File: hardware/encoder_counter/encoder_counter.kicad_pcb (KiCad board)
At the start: 2 copper layers, 32 parts, among them P1 5045-3, P2 FEMALE_HEADER, P3 5045-3, P4 5045-3, P5 FEMALE_HEADER, P6 FEMALE_HEADER, P7 5045-3, P8 FEMALE_HEADER, P9 FEMALE_HEADER, U5 LS7366R, U6 LS7366R, Y1 32 MHz, Y2 32 MHz

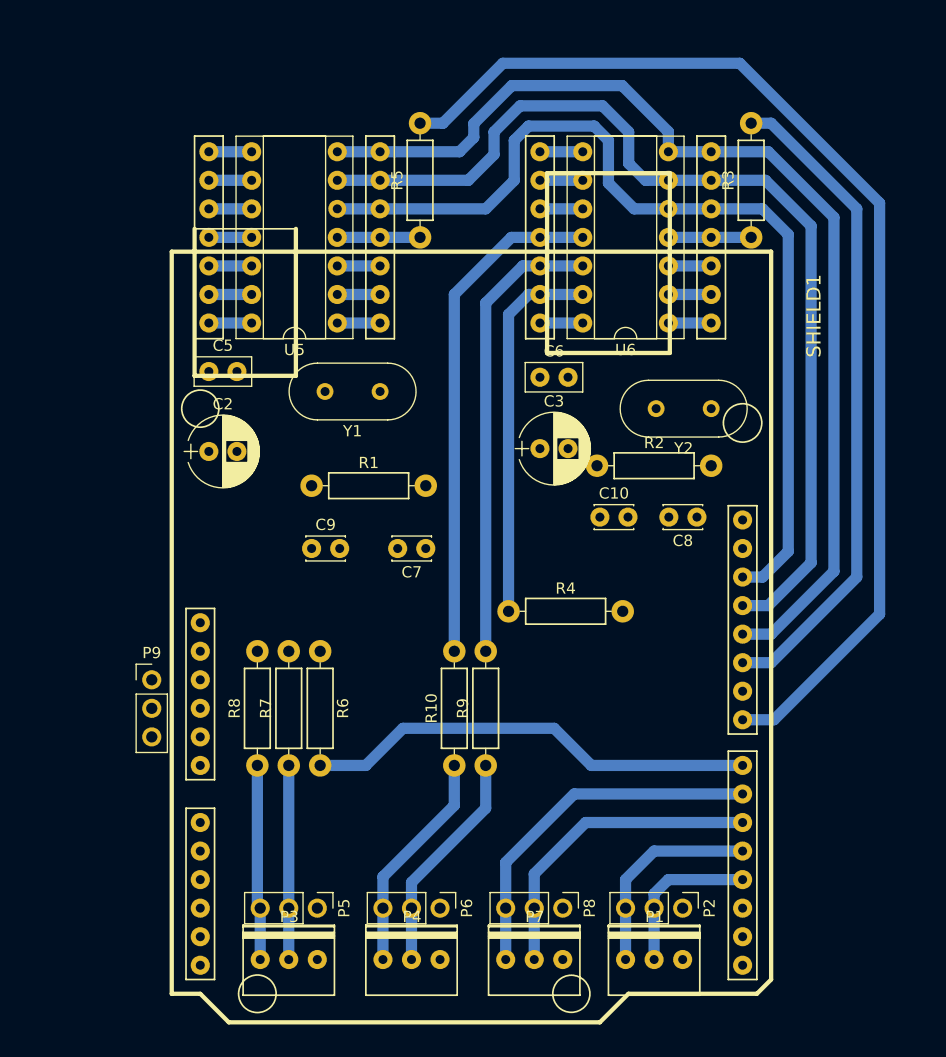
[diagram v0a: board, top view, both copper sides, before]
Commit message: Last version.
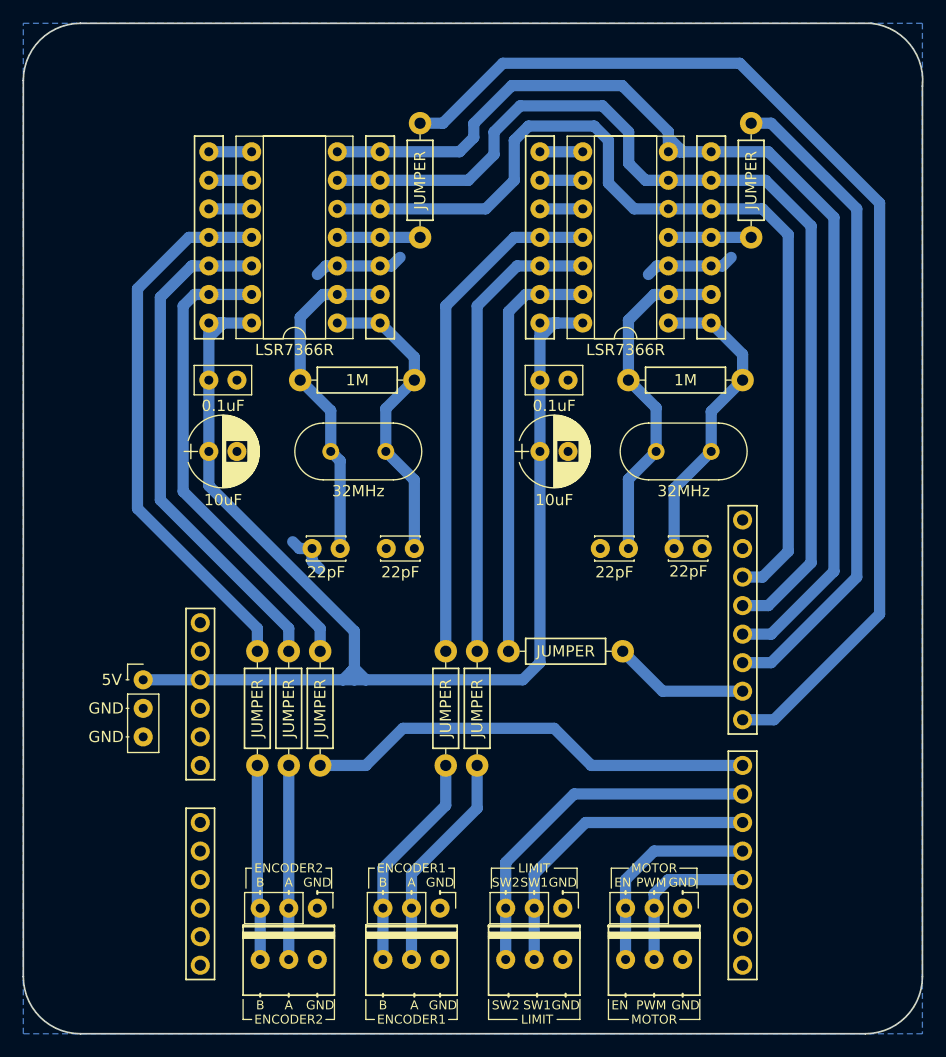
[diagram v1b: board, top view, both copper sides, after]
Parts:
- P2, P5, P6, P8, P9: footprint Maplex_Misc:Pin_Header_Straight_1x03_Pitch2.54mm -> Maplex_Misc:Female_Header_Straight_1x03_Pitch2.54mm
- moved 1M 9.45 mm to (86.6, 83.1)
- moved 1M 8.12 mm to (115.8, 83.1)
- moved 32MHz 5.36 mm to (94.2, 89.4)
- moved 32MHz 3.81 mm to (123.2, 89.4)
- moved 22pF 3.78 mm to (115.8, 98.0), turned to 180 degrees
- moved JUMPER 3.56 mm to (105.2, 107.2)
- moved 22pF 3.45 mm to (119.9, 98.0), turned to 0 degrees
- moved 22pF 2.54 mm to (90.2, 98.0), turned to 180 degrees
- moved 22pF 1.02 mm to (96.8, 98.0)
- moved 0.1uF 0.76 mm to (78.5, 83.1)
- moved JUMPER 0.76 mm to (102.4, 117.3)
- moved JUMPER 0.76 mm to (99.6, 117.3)
- moved P9 0.76 mm to (72.6, 109.7)
- moved 0.1uF 0.25 mm to (108.0, 83.1)
- moved 10uF 0.25 mm to (108.0, 89.4)
- renumbered C5 to 0.1uF, C6 to 0.1uF, C2 to 10uF, C3 to 10uF, R1 to 1M, R2 to 1M, C7 to 22pF, C8 to 22pF, C9 to 22pF, C10 to 22pF, Y2 to 32MHz, Y1 to 32MHz, R3 to JUMPER, R4 to JUMPER, R5 to JUMPER, R6 to JUMPER, R7 to JUMPER, R8 to JUMPER, R9 to JUMPER, R10 to JUMPER, U5 to LSR7366R, U6 to LSR7366R
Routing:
- net +5V: track 7.62 -> 118.8 mm
- net Net-(R8-Pad2): track 3.81 -> 48.7 mm
- net Net-(R7-Pad2): track 3.81 -> 45.5 mm
- net EN_C1: track 3.81 -> 42.3 mm
- net Net-(C10-Pad1): track 3.81 -> 30.7 mm
- net Net-(C9-Pad1): track 3.81 -> 30.0 mm
- net Net-(C8-Pad1): track 3.81 -> 27.6 mm
- net Net-(C7-Pad1): track 3.81 -> 27.2 mm
- net GND: track 7.62 -> 20.1 mm
- net Net-(R4-Pad2): track 0.00 -> 12.1 mm
- net EN_C2: track 33.8 -> 37.5 mm
- net MOSI: track 95.2 -> 97.6 mm
- net Net-(R9-Pad2): track 41.0 -> 41.6 mm
- added copper zone on B.Cu, net GND
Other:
- board outline added: 80 x 89.9 mm
- net class Default: clearance 0.8 -> 0.75
- rule trace_clearance: 0.8 -> 0.75
- board text added: "5V"
- board text added: "A"
- board text added: "B"
- board text added: "EN"
- board text added: "ENCODER1"
- board text added: "ENCODER2"
- board text added: "GND"
- board text added: "LIMIT"
- board text added: "MOTOR"
- board text added: "PWM"
- board text added: "SW1"
- board text added: "SW2"
